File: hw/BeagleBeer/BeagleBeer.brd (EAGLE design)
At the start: 130.8 x 118.7 mm, 99 parts, among them U1 TEMPERATURE-SENSORUMAX8, U5 CAT24C256WI-GT3

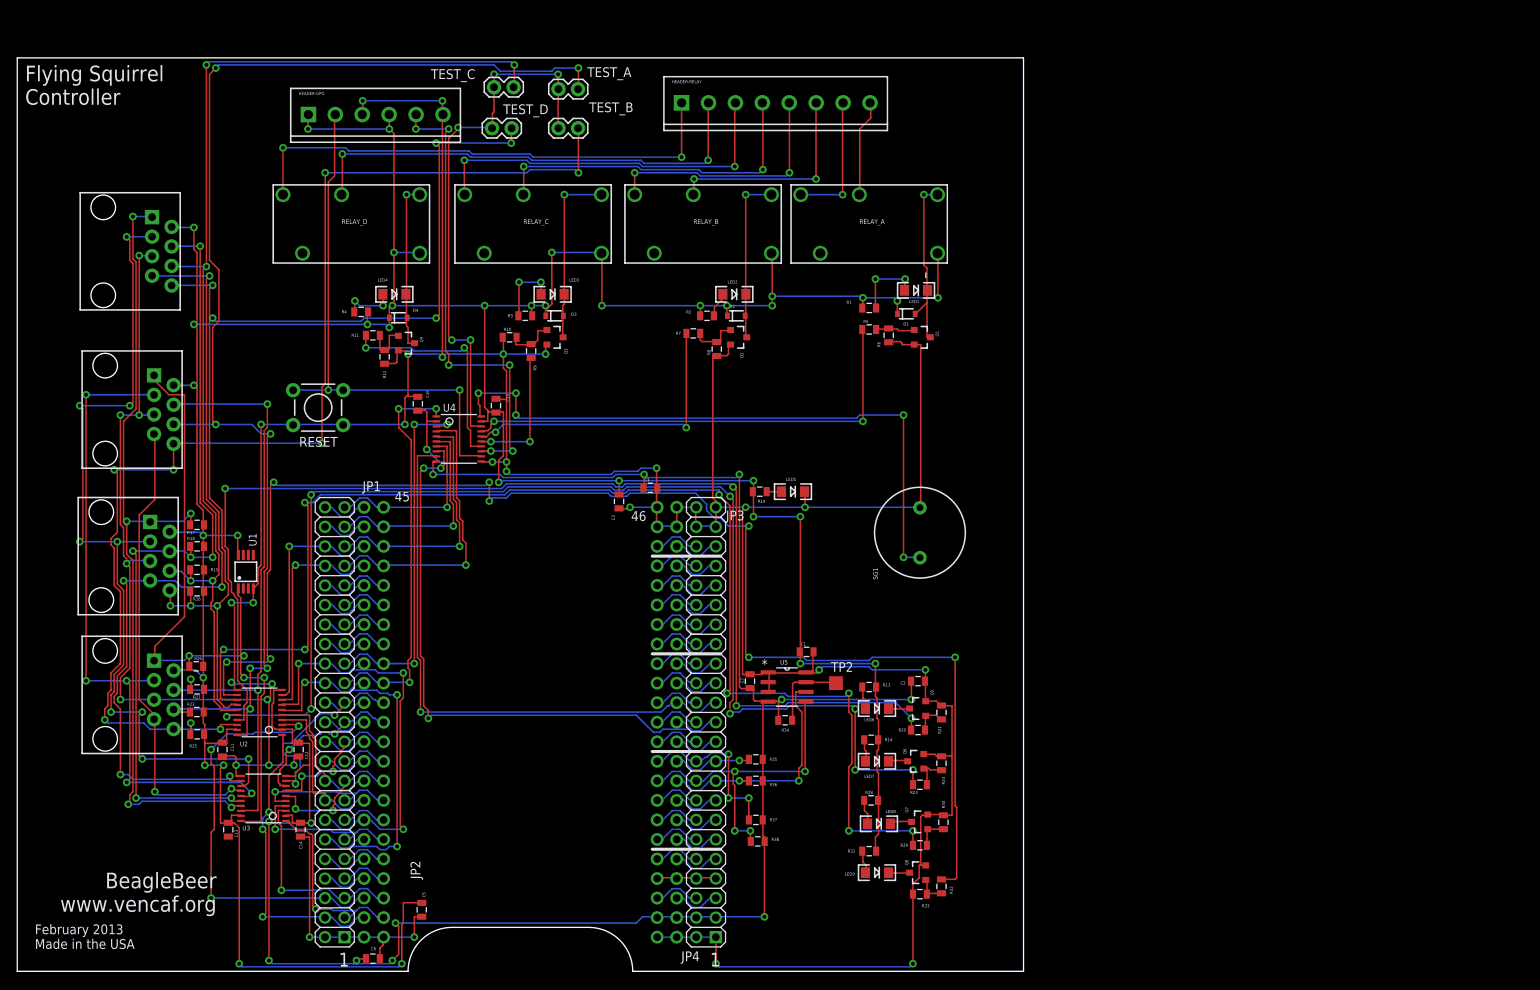
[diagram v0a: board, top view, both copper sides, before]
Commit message: Clean up Gerber files.  Generate XY parts placement files.
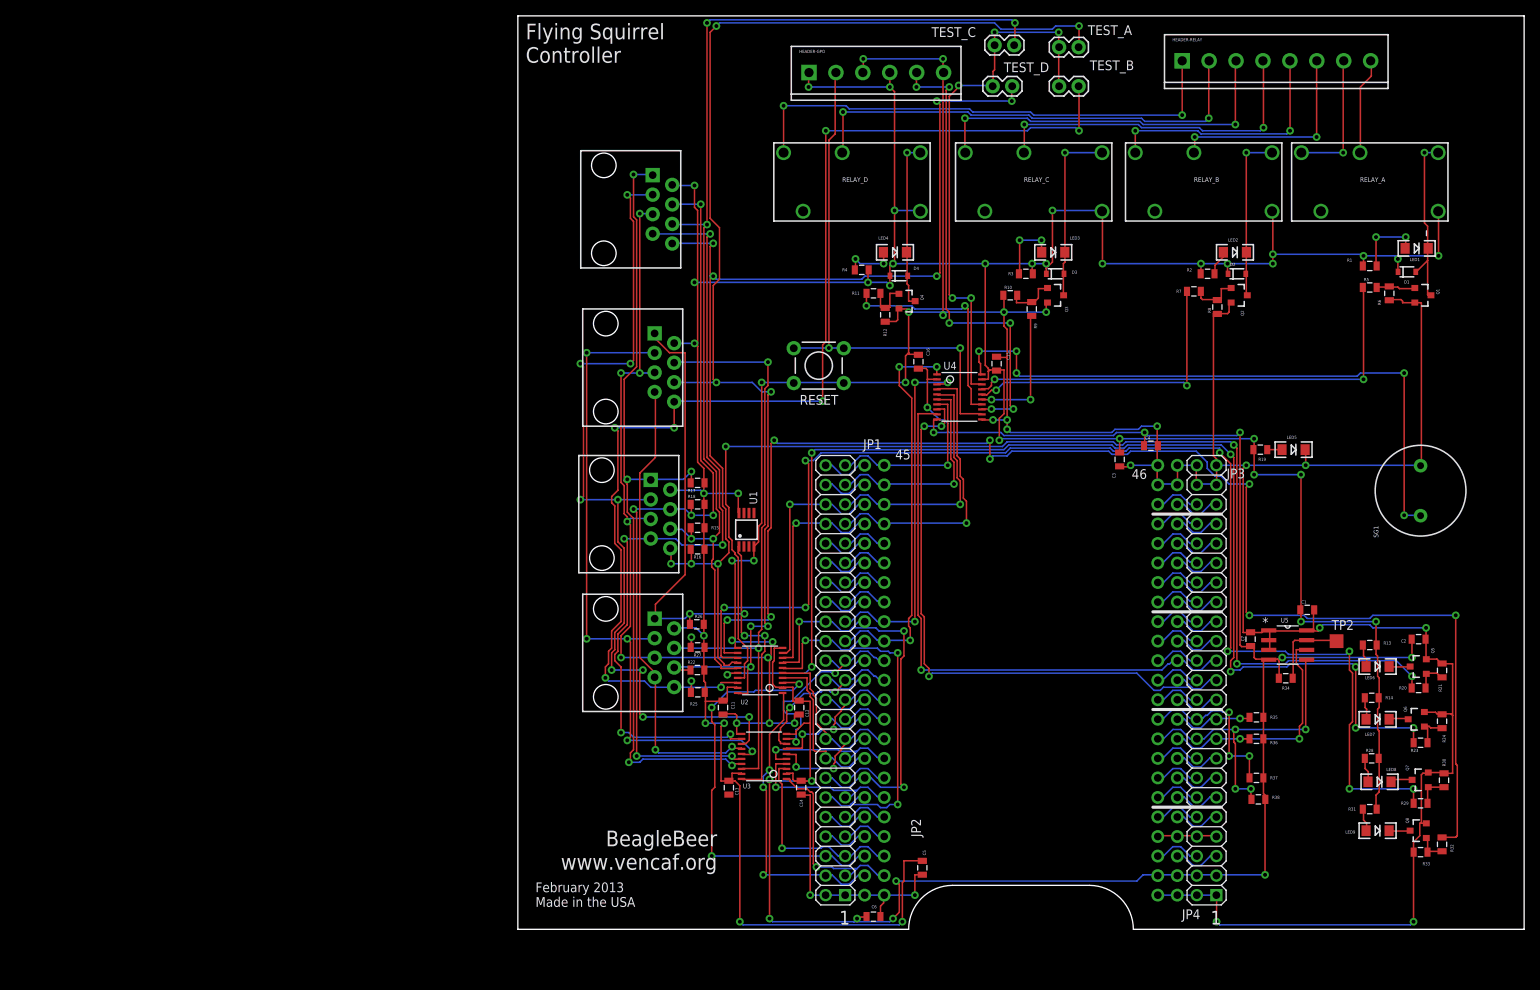
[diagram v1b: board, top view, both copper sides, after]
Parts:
- moved C12 65.3 mm to (36.6, 28.8)
- moved C16 65.3 mm to (52.1, 73.8)
- moved C2 65.3 mm to (117.1, 37.7)
- moved C4 65.3 mm to (82.3, 62.9)
- moved D1 65.3 mm to (115.6, 85.5)
- moved D2 65.3 mm to (93.5, 85.2)
- moved D3 65.3 mm to (69.9, 85.2)
- moved D4 65.3 mm to (49.6, 85.0)
- moved JP1 65.3 mm to (47.7, 32.4)
- moved JP2 65.3 mm to (45.1, 32.4)
- moved JP3 65.3 mm to (85.8, 32.4)
- moved LED5 65.3 mm to (100.9, 62.4)
- moved LED6 65.3 mm to (111.8, 34.2)
- moved LED7 65.3 mm to (111.8, 27.3)
- moved LED8 65.3 mm to (112.1, 19.2)
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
